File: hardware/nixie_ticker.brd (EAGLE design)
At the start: 127 x 61 mm, 62 parts, among them Q1 BCX19SMD, Q2 BCX19SMD

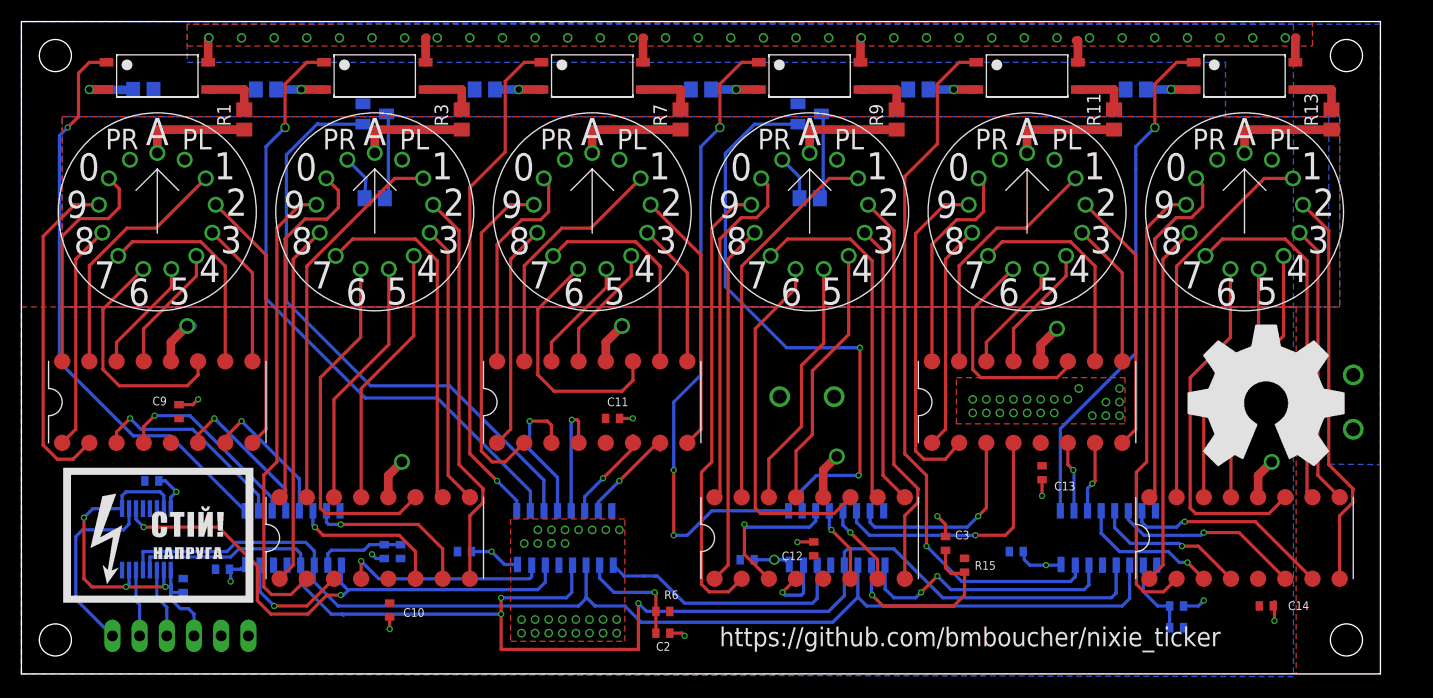
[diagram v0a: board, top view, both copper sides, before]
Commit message: Updates 7-7
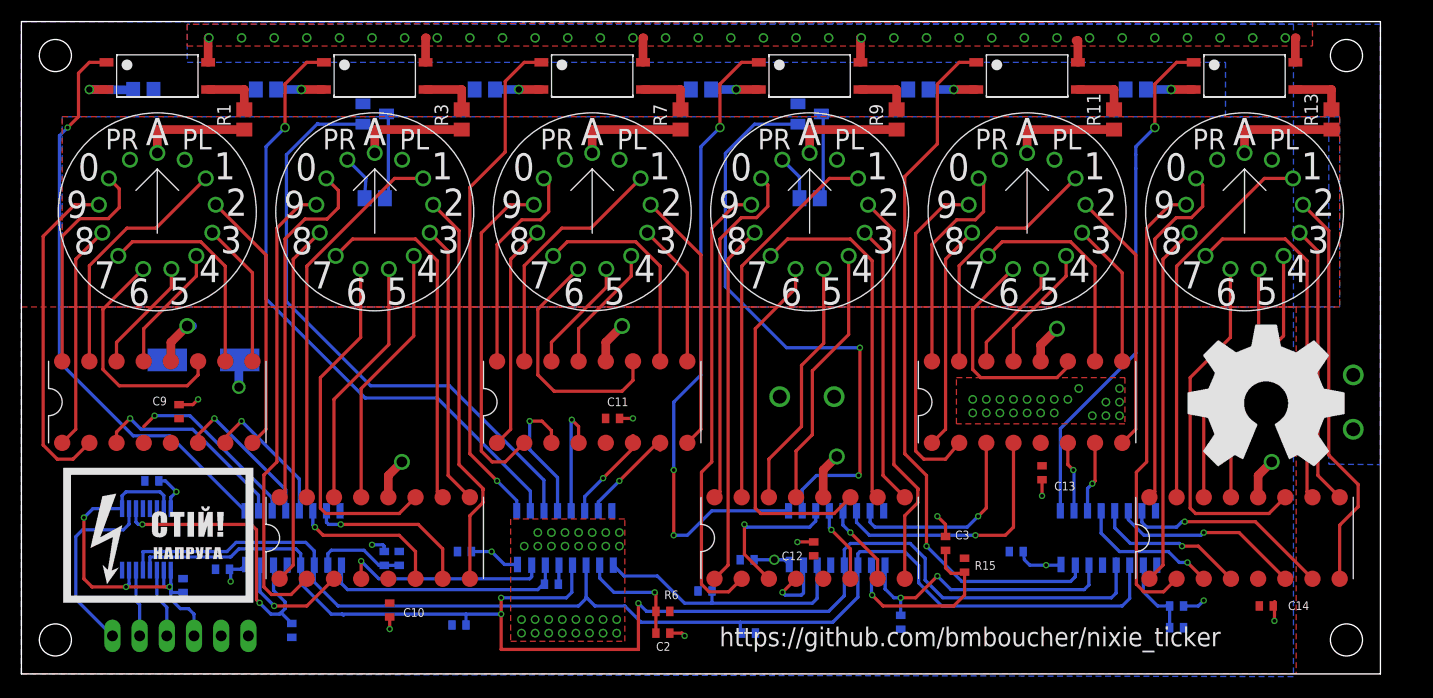
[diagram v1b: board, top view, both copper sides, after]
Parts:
- added CD40109B: CD40109B, nixie_ticker:SOP65P640X120-16
- added R19, R20, R21, R22, R23, R24: (no value), resistor:R0402
- U$25: value CD40109B -> UUR1C221MCL6GS; device nixie_ticker:SOP65P640X120-16 -> nixie_ticker:CAPAE830X1050
- moved U$25 17.6 mm to (17.0, 29.3), turned to 0 degrees
- moved C1 0.65 mm to (35.3, 10.8), turned to 90 degrees
- moved R5 0.63 mm to (33.9, 10.8), turned to 90 degrees
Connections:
- removed net N$152: JP1.4, U$25.3
- removed net N$159: JP1.6, U$25.10
- removed net N$86: U$10.P$12, U$25.4, U$3.P$12, U$4.P$12, U$9.P$12
- removed net N$87: U$10.P$11, U$25.5, U$3.P$11, U$4.P$11, U$9.P$11
- removed net N$88: JP1.5, U$25.6
- new net DI_L: CD40109B.10, JP1.6
- new net DS_1: CD40109B.11, R21.2, U$3.P$14
- new net SHCP_5V: CD40109B.5, R19.2, U$10.P$11, U$3.P$11, U$4.P$11, U$9.P$11
- new net SHCP_L: CD40109B.6, JP1.5
- new net STCP_5V: CD40109B.4, R20.2, U$10.P$12, U$3.P$12, U$4.P$12, U$9.P$12
- new net STCP_L: CD40109B.3, JP1.4
- net +3V3: now also CD40109B.1, CD40109B.15, CD40109B.2, CD40109B.7, CD40109B.9; no longer U$25.1, U$25.15, U$25.2, U$25.7, U$25.9
- net +5V: now also CD40109B.16, U$25.1; no longer U$25.16
- net GND: now also CD40109B.8, R19.1, R20.1, R21.1, R22.1, R23.1, R24.1, U$25.2; no longer U$25.8
- net N$21: now also R23.2
- net N$22: now also R22.2; no longer U$25.11
- net N$23: now also R24.2
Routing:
- net STCP_5V: track 0.00 -> 127.9 mm, vias 0 -> 3
- net N$86: track 125.1 -> 0.00 mm, vias 3 -> 0
- net SHCP_5V: track 0.00 -> 115.4 mm
- net N$87: track 110.5 -> 0.00 mm
- net DS_1: track 0.00 -> 28.7 mm, vias 0 -> 2
- net N$22: track 50.3 -> 23.0 mm, vias 2 -> 0
- net N$159: track 17.6 -> 0.00 mm
- net DI_L: track 0.00 -> 17.6 mm
- net STCP_L: track 0.00 -> 6.53 mm
- net N$152: track 6.53 -> 0.00 mm
- net SHCP_L: track 0.00 -> 6.29 mm
- net N$88: track 6.29 -> 0.00 mm
- net +5V: track 22.9 -> 25.9 mm, vias 7 -> 8
- net GND: track 37.3 -> 39.1 mm, vias 63 -> 67
- net N$23: track 25.0 -> 26.6 mm
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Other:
- board text added: "3V3"
- board text added: "5V"
- board text added: "DI"
- board text added: "GND"
- board text added: "SHCP"
- board text added: "STCP"

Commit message: Updating 8-12
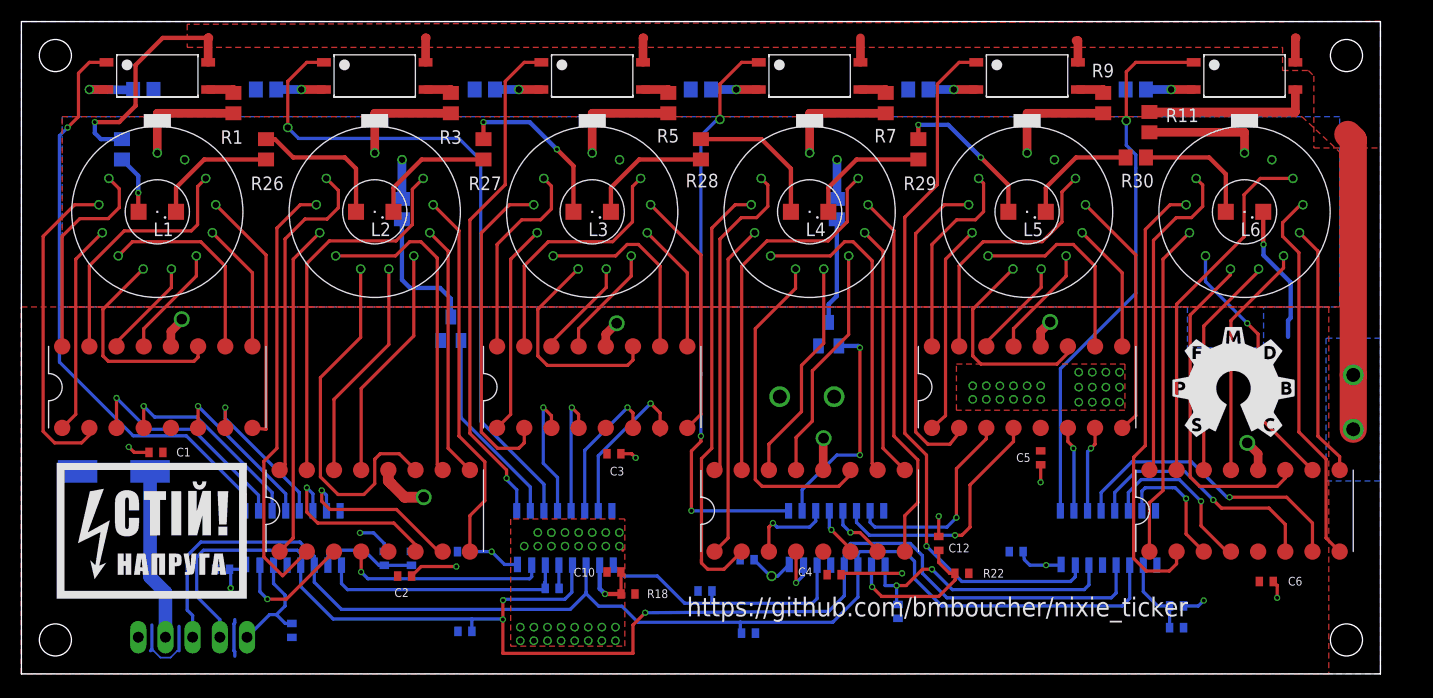
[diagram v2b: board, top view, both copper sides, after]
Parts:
- removed C16: (no value), resistor:C0402
- removed CD40109B: CD40109B, nixie_ticker:SOP65P640X120-16
- removed JP1: (no value), pinhead:1X06
- removed U$1, U$11, U$15, U$19, U$2, U$5: IN14, nixie_ticker:IN14
- removed U$12, U$16, U$20, U$6, U$7, U$8: K155ID1, nixie_ticker:DIP-16_SMD
- removed U$25: UUR1C221MCL6GS, nixie_ticker:CAPAE830X1050
- added JP2: (no value), pinhead:1X05
- added L1, L2, L3, L4, L5, L6: (no value), led:SML1206
- added N1, N2, N3, N4, N5, N6: IN14_12PIN12PIN, nixie_ticker:IN14-12PIN
- added R25, R26, R27, R28, R29, R30: (no value), resistor:R0805
- added U1, U2, U3, U4, U5, U6: K155ID1, nixie_ticker:DIP-16_SMD
- C15: value (none) -> 220uF; device resistor:C0402 -> nixie_ticker:CAPAE830X1050
- R17, R18: device resistor:R0805 -> resistor:R0402
- R5, R6: device resistor:R0402 -> resistor:R0805
- moved R13 87.3 mm to (35.6, 43.4), flipped to the bottom
- moved R16 82.7 mm to (25.3, 4.06), turned to 90 degrees
- moved C7 74.2 mm to (18.8, 9.78)
- moved C8 71.8 mm to (36.4, 10.8), turned to 90 degrees
- moved C4 57.2 mm to (75.9, 9.27), flipped to the top
- moved C5 54.6 mm to (95.2, 20.2), flipped to the top, turned to 270 degrees
- moved R15 54.2 mm to (33.9, 10.8), flipped to the bottom
- moved R6 51.5 mm to (43.3, 54.6), flipped to the bottom, turned to 180 degrees
- moved R5 50.1 mm to (60.5, 53.3), flipped to the top
- moved C6 48.6 mm to (116.3, 8.64), flipped to the top
- moved R18 43.9 mm to (56.7, 7.47), flipped to the top
- moved R17 43.7 mm to (49.6, 7.99)
- moved R21 38.8 mm to (63.9, 7.75), turned to 180 degrees
- moved R22 38.4 mm to (87.9, 9.40), flipped to the top
- moved C3 32.1 mm to (55.4, 20.6), turned to 0 degrees
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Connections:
- net N$28 renamed D1A
- net N$49 renamed D3A
- net N$55 renamed D4PR
- net N$56 renamed D4A
- net N$60 renamed D5A
- net N$85 renamed D6A
- removed net +3V3: C16.1, CD40109B.1, CD40109B.15, CD40109B.2, CD40109B.7, CD40109B.9, JP1.3
- removed net DI_L: CD40109B.10, JP1.6
- removed net DS_1: CD40109B.11, R21.2, U$3.P$14
- removed net N$101: U$10.P$2, U$16.P$6
- removed net N$45: U$4.P$6, U$6.P$6
- removed net N$46: U$4.P$7, U$6.P$7
- removed net N$47: U$4.P$15, U$8.P$4
- removed net N$48: U$4.P$5, U$6.P$4
- removed net N$50: U$12.P$3, U$9.P$3
- removed net N$51: U$12.P$6, U$9.P$4
- removed net N$52: U$12.P$7, U$9.P$5
- removed net N$53: U$12.P$4, U$9.P$15
- removed net N$54: U$16.P$3, U$9.P$7
- removed net N$58: U$10.P$3, U$16.P$7
- removed net N$59: U$16.P$4, U$9.P$6
- removed net N$81: U$10.P$4, U$20.P$3
- removed net N$82: U$10.P$6, U$20.P$6
- removed net N$83: U$10.P$7, U$20.P$7
- removed net N$84: U$10.P$5, U$20.P$4
- removed net SHCP_5V: CD40109B.5, R19.2, U$10.P$11, U$3.P$11, U$4.P$11, U$9.P$11
- removed net SHCP_L: CD40109B.6, JP1.5
- removed net STCP_5V: CD40109B.4, R20.2, U$10.P$12, U$3.P$12, U$4.P$12, U$9.P$12
- removed net STCP_L: CD40109B.3, JP1.4
- new net CLK: JP2.4, R20.2, U$10.P$12, U$3.P$12, U$4.P$12, U$9.P$12
- new net D1I1: U$3.P$2, U1.P$3
- new net D1I2: U$3.P$4, U1.P$6
- new net D1I4: U$3.P$5, U1.P$7
- new net D1I8: U$3.P$3, U1.P$4
- new net D2A: U$14.1, U$4.P$3
- new net D2I1: U$3.P$15, U2.P$3
- new net D2I2: U$3.P$6, U2.P$6
- new net D2I4: U$3.P$7, U2.P$7
- new net D2I8: U$4.P$15, U2.P$4
- new net D2PR: Q1.B, U$4.P$2
- new net D3I1: U$4.P$4, U3.P$3
- new net D3I2: U$4.P$6, U3.P$6
- new net D3I4: U$4.P$7, U3.P$7
- new net D3I8: U$4.P$5, U3.P$4
- new net D4I1: U$9.P$3, U4.P$3
- new net D4I2: U$9.P$4, U4.P$6
- new net D4I4: U$9.P$5, U4.P$7
- new net D4I8: U$9.P$15, U4.P$4
- new net D5I1: U$9.P$7, U5.P$3
- new net D5I2: U$10.P$2, U5.P$6
- new net D5I4: U$10.P$3, U5.P$7
- new net D5I8: U$9.P$6, U5.P$4
- new net D6I1: U$10.P$7, U6.P$3
- new net D6I2: U$10.P$5, U6.P$6
- new net D6I4: U$10.P$4, U6.P$7
- new net D6I8: U$10.P$6, U6.P$4
- new net DATA: JP2.5, R16.2, U$3.P$14
- new net LATCH: JP2.3, R19.2, U$10.P$11, U$3.P$11, U$4.P$11, U$9.P$11
- new net N$28: L3.C, R28.1
- net +5V: now also C1.1, C2.1, C3.1, JP2.2, R18.2, R22.2, R24.2, U1.P$5, U2.P$5, U3.P$5, U4.P$5, U5.P$5, U6.P$5; no longer C10.1, C12.1, C14.1, CD40109B.16, JP1.2, R16.2, R5.2, R6.2, U$12.P$5, U$16.P$5, U$20.P$5, U$25.1, U$6.P$5, U$7.P$5, U$8.P$5
- net GND: now also JP2.1, L6.C, R16.1, R17.1, R6.1, U1.P$12, U2.P$12, U3.P$12, U4.P$12, U5.P$12, U6.P$12; no longer C16.2, CD40109B.8, JP1.1, R14.1, R22.1, R24.1, U$12.P$12, U$16.P$12, U$20.P$12, U$25.2, U$6.P$12, U$7.P$12, U$8.P$12
- net N$1: now also N1.P$12, U1.P$16; no longer U$1.P$12, U$7.P$16
- net N$10: now also N1.P$11, U1.P$2; no longer U$1.P$11, U$7.P$2
- net N$100: now also N5.P$11, U5.P$2; no longer U$15.P$11, U$16.P$2
- net N$104: now also N6.P$1, R11.1; no longer R13.1, U$19.P$1
- net N$105: now also N2.P$1; no longer U$2.P$1
- net N$108: now also C10.1, R18.1; no longer C2.1, R6.1
- net N$109: now also C8.1, R15.1; no longer C1.1, R5.1
- net N$11: now also N2.P$12, U2.P$16; no longer U$2.P$12, U$8.P$16
- net N$110: now also C12.1, R22.1; no longer C3.1, R15.1
- net N$111: now also C14.1, R24.1; no longer C8.1, R16.1
- net N$112: now also R5.2; no longer R7.2
- net N$113: now also R6.2; no longer R8.2
- net N$118: now also N3.P$1, R5.1; no longer R7.1, U$5.P$1
- net N$119: now also R7.2; no longer R9.2
- net N$12: now also N2.P$3, U2.P$15; no longer U$2.P$3, U$8.P$15
- net N$120: now also R8.2; no longer R10.2
- net N$121: now also N6.P$12, U6.P$16; no longer U$19.P$12, U$20.P$16
- net N$122: now also N6.P$3, U6.P$15; no longer U$19.P$3, U$20.P$15
- net N$123: now also N6.P$4, U6.P$8; no longer U$19.P$4, U$20.P$8
- net N$124: now also N6.P$5, U6.P$9; no longer U$19.P$5, U$20.P$9
- net N$125: now also N6.P$6, U6.P$13; no longer U$19.P$6, U$20.P$13
- net N$126: now also N6.P$7, U6.P$14; no longer U$19.P$7, U$20.P$14
- net N$127: now also N6.P$8, U6.P$11; no longer U$19.P$8, U$20.P$11
- net N$128: now also N6.P$9, U6.P$10; no longer U$19.P$9, U$20.P$10
- net N$129: now also N6.P$10, U6.P$1; no longer U$19.P$10, U$20.P$1
- net N$13: now also N2.P$4, U2.P$8; no longer U$2.P$4, U$8.P$8
- net N$130: now also N6.P$11, U6.P$2; no longer U$19.P$11, U$20.P$2
- net N$14: now also N2.P$5, U2.P$9; no longer U$2.P$5, U$8.P$9
- net N$145: now also N4.P$1, R7.1; no longer R9.1, U$11.P$1
- net N$146: now also R9.2; no longer R11.2
- net N$147: now also R10.2; no longer R12.2
- net N$15: now also N2.P$6, U2.P$13; no longer U$2.P$6, U$8.P$13
- net N$153: now also R11.2; no longer R13.2
- net N$154: now also R12.2; no longer R14.2
- net N$16: now also N2.P$7, U2.P$14; no longer U$2.P$7, U$8.P$14
- net N$160: now also R13.1; no longer R18.1
- net N$161: now also R14.1; no longer R17.1
- net N$162: now also N4.P$2, R14.2; no longer R17.2, U$11.P$13
- net N$163: now also N2.P$2, R13.2; no longer R18.2, U$2.P$13
- net N$17: now also N2.P$8, U2.P$11; no longer U$2.P$8, U$8.P$11
- net N$18: now also N2.P$9, U2.P$10; no longer U$2.P$9, U$8.P$10
- net N$19: now also N2.P$10, U2.P$1; no longer U$2.P$10, U$8.P$1
- net N$2: now also N1.P$3, U1.P$15; no longer U$1.P$3, U$7.P$15
- net N$20: now also N2.P$11, U2.P$2; no longer U$2.P$11, U$8.P$2
- net N$21: now also R21.2; no longer R23.2
- net N$22: now also R17.2; no longer R22.2
- net N$23: now also R23.2; no longer R24.2
- net N$24: now also L1.C, R26.1; no longer U$3.P$2, U$7.P$3
- net N$25: now also L2.A, R26.2; no longer U$3.P$4, U$7.P$6
- net N$26: now also L2.C, R27.2; no longer U$3.P$5, U$7.P$7
- net N$27: now also L3.A, R27.1; no longer U$3.P$3, U$7.P$4
- net N$29: now also L1.A, R25.1; no longer U$3.P$15, U$8.P$3
- net N$3: now also N1.P$4, U1.P$8; no longer U$1.P$4, U$7.P$8
- net N$30: now also L4.A, R28.2; no longer U$3.P$6, U$8.P$6
- net N$31: now also N3.P$12, U3.P$16; no longer U$5.P$12, U$6.P$16
- net N$32: now also N3.P$3, U3.P$15; no longer U$5.P$3, U$6.P$15
- net N$33: now also N3.P$4, U3.P$8; no longer U$5.P$4, U$6.P$8
- net N$34: now also N3.P$5, U3.P$9; no longer U$5.P$5, U$6.P$9
- net N$35: now also N3.P$6, U3.P$13; no longer U$5.P$6, U$6.P$13
- net N$36: now also N3.P$7, U3.P$14; no longer U$5.P$7, U$6.P$14
- net N$37: now also N3.P$8, U3.P$11; no longer U$5.P$8, U$6.P$11
- net N$38: now also N3.P$9, U3.P$10; no longer U$5.P$9, U$6.P$10
- net N$39: now also N3.P$10, U3.P$1; no longer U$5.P$10, U$6.P$1
- net N$4: now also N1.P$5, U1.P$9; no longer U$1.P$5, U$7.P$9
- net N$40: now also N3.P$11, U3.P$2; no longer U$5.P$11, U$6.P$2
- net N$41: now also L4.C, R29.2; no longer U$3.P$7, U$8.P$7
- net N$42: now also L5.A, R29.1; no longer Q1.B, U$4.P$3
- net N$43: now also L5.C, R30.1; no longer U$14.1, U$4.P$2
- net N$44: now also L6.A, R30.2; no longer U$4.P$4, U$6.P$3
- net N$5: now also N1.P$6, U1.P$13; no longer U$1.P$6, U$7.P$13
- net N$57: now also N1.P$1; no longer U$1.P$1
- net N$6: now also N1.P$7, U1.P$14; no longer U$1.P$7, U$7.P$14
- net N$61: now also N4.P$12, U4.P$16; no longer U$11.P$12, U$12.P$16
- net N$62: now also N4.P$3, U4.P$15; no longer U$11.P$3, U$12.P$15
- net N$63: now also N4.P$4, U4.P$8; no longer U$11.P$4, U$12.P$8
- net N$64: now also N4.P$5, U4.P$9; no longer U$11.P$5, U$12.P$9
- net N$65: now also N4.P$6, U4.P$13; no longer U$11.P$6, U$12.P$13
- net N$66: now also N4.P$7, U4.P$14; no longer U$11.P$7, U$12.P$14
- net N$67: now also N4.P$8, U4.P$11; no longer U$11.P$8, U$12.P$11
- net N$68: now also N4.P$9, U4.P$10; no longer U$11.P$9, U$12.P$10
- net N$69: now also N4.P$10, U4.P$1; no longer U$11.P$10, U$12.P$1
- net N$7: now also N1.P$8, U1.P$11; no longer U$1.P$8, U$7.P$11
- net N$70: now also N4.P$11, U4.P$2; no longer U$11.P$11, U$12.P$2
- net N$8: now also N1.P$9, U1.P$10; no longer U$1.P$9, U$7.P$10
- net N$9: now also N1.P$10, U1.P$1; no longer U$1.P$10, U$7.P$1
- net N$90: now also N5.P$1, R9.1; no longer R11.1, U$15.P$1
- net N$91: now also N5.P$12, U5.P$16; no longer U$15.P$12, U$16.P$16
- net N$92: now also N5.P$3, U5.P$15; no longer U$15.P$3, U$16.P$15
- net N$93: now also N5.P$4, U5.P$8; no longer U$15.P$4, U$16.P$8
- net N$94: now also N5.P$5, U5.P$9; no longer U$15.P$5, U$16.P$9
- net N$95: now also N5.P$6, U5.P$13; no longer U$15.P$6, U$16.P$13
- net N$96: now also N5.P$7, U5.P$14; no longer U$15.P$7, U$16.P$14
- net N$97: now also N5.P$8, U5.P$11; no longer U$15.P$8, U$16.P$11
- net N$98: now also N5.P$9, U5.P$10; no longer U$15.P$9, U$16.P$10
- net N$99: now also N5.P$10, U5.P$1; no longer U$15.P$10, U$16.P$1
- net V+: now also R25.2
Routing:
- net CLK: track 0.00 -> 129.2 mm, vias 0 -> 3
- net STCP_5V: track 127.9 -> 0.00 mm, vias 3 -> 0
- net LATCH: track 0.00 -> 117.5 mm
- net SHCP_5V: track 115.4 -> 0.00 mm
- net D2A: track 0.00 -> 62.9 mm, vias 0 -> 1
- net N$43: track 59.3 -> 10.9 mm, vias 1 -> 0
- net V+: track 14.1 -> 61.7 mm, vias 34 -> 1
- net N$42: track 55.9 -> 14.6 mm, vias 0 -> 2
- net +3V3: track 38.6 -> 0.00 mm, vias 3 -> 0
- net D4PR: track 55.1 -> 20.8 mm
- net DS_1: track 28.7 -> 0.00 mm, vias 2 -> 0
- net D6I4: track 0.00 -> 27.7 mm, vias 0 -> 1
- net GND: track 39.1 -> 64.8 mm, vias 67 -> 69
- net N$59: track 24.4 -> 0.00 mm, vias 1 -> 0
- net D5I8: track 0.00 -> 23.5 mm, vias 0 -> 1
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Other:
- board text added: "00 D6 1 08 D5 1 16 D3 4 24 D2 4 01 D6 8 09 D5 8 17 D3 2 25 D2 2 02 D6 2 10 D4 4 18 D3 8 26 D1 4 03 D6 4 11 D4 2 19 D3 1 27 D1 2 04 D5 4 12 D4 1 20 D2 A 28 D1 8 05 D5 2 13 D4 P 21 D2 P 29 D1 1 06 D6 A 14 D4 A 22 D3 A 30 D1 A 07 D5 A 15 D4 8 23 D2 8 31 D2 1"
- board text added: "C"
- board text added: "D"
- board text added: "D1"
- board text added: "D2"
- board text added: "D3"
- board text added: "D4"
- board text added: "D5"
- board text added: "D6"
- board text added: "L"
- board text added: "POS"
- board text removed: "3V3"
- board text removed: "DI"
- board text removed: "SHCP"
- board text removed: "STCP"
